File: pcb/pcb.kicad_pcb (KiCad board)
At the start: 2 copper layers, 100 x 115 mm, 27 parts, among them J1 Screw_Terminal_01x02, J2 Screw_Terminal_01x04, J3 Screw_Terminal_01x04, J5 Screw_Terminal_01x06, J6 Screw_Terminal_01x04, Q1 2N7000, Q2 2N7000, Q3 2N7000

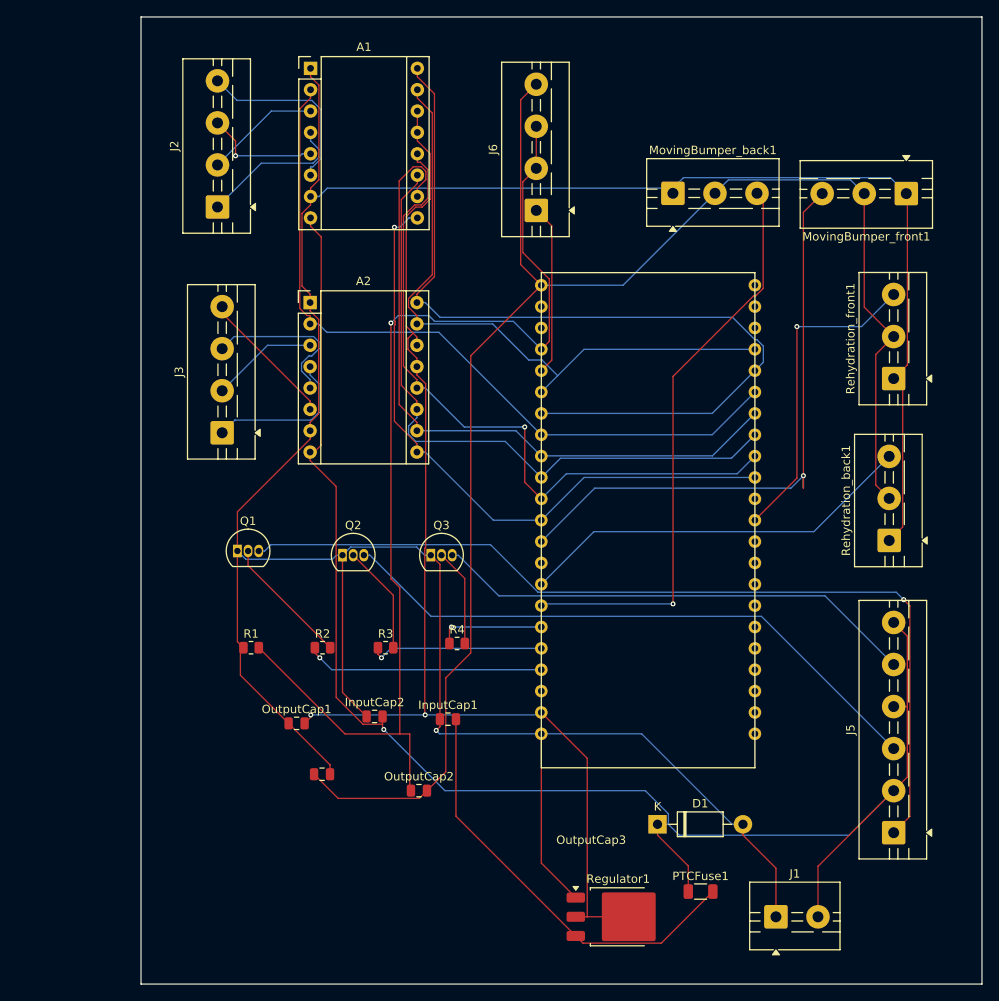
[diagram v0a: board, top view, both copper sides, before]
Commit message: finished layout
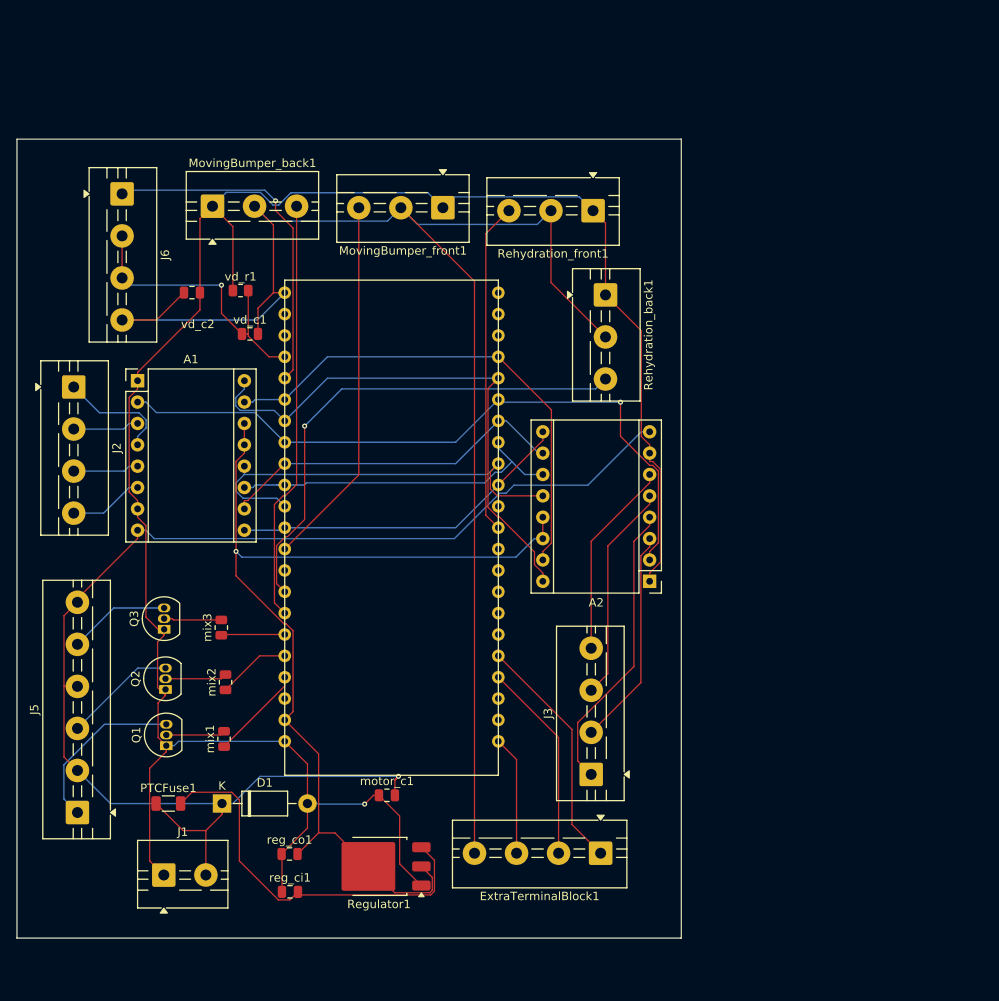
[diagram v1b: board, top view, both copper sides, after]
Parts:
- added ExtraTerminalBlock1: Screw_Terminal_01x04, TerminalBlock:TerminalBlock_MaiXu_MX126-5.0-04P_1x04_P5.00mm, F.Cu at (166.2, 134.4)
- moved J5 97.1 mm to (103.9, 129.6)
- moved J1 73.0 mm to (114.2, 137.0)
- moved PTCFuse1 64.1 mm to (114.8, 128.5)
- moved J3 59.8 mm to (165.0, 125.1)
- moved vd_c2 59.3 mm to (117.6, 67.8)
- moved vd_c1 57.9 mm to (124.5, 72.7)
- moved MovingBumper_front1 55.1 mm to (147.4, 57.7)
- moved MovingBumper_back1 54.8 mm to (120.0, 57.5)
- moved A2 52.2 mm to (172.0, 102.1), turned to 180 degrees
- moved D1 51.8 mm to (121.1, 128.5)
- moved J6 49.3 mm to (109.2, 56.0), turned to -90 degrees
- moved Rehydration_back1 44.6 mm to (166.7, 68.0), turned to -90 degrees
- moved vd_r1 42.5 mm to (123.3, 67.5)
- moved A1 42.5 mm to (111.1, 78.3)
- moved Rehydration_front1 40.9 mm to (165.2, 58.0), turned to 180 degrees
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- renumbered R2 to mix1, R3 to mix2, R4 to mix3, InputCap2 to motor_c1, InputCap1 to reg_ci1, OutputCap1 to reg_co1, OutputCap2 to vd_c1, OutputCap3 to vd_c2, R1 to vd_r1
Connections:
- ESP32-S3 pad 40: unconnected-(ESP32-S3-21-Pad40) -> Net-(ESP32-S3-21)
- ESP32-S3 pad 41: unconnected-(ESP32-S3-20-Pad41) -> Net-(ESP32-S3-20)
- ESP32-S3 pad 44: unconnected-(ESP32-S3-GND-Pad44) -> Net-(ExtraTerminalBlock1-Pin_3)
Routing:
- net Net-(D1-A): track 352.5 -> 254.5 mm
- net /VD_o: track 127.1 -> 35.5 mm
- net Net-(J5-Pin_1): track 108.5 -> 20.5 mm, vias 1 -> 0
- net Net-(J5-Pin_3): track 72.5 -> 13.4 mm
- net Net-(J5-Pin_5): track 57.9 -> 12.1 mm
- net /M0: track 81.6 -> 42.0 mm
- net /DIR: track 103.7 -> 65.0 mm
- net /M1: track 78.2 -> 41.3 mm
- net /EN: track 76.8 -> 40.9 mm, vias 1 -> 0
- net /M2: track 82.5 -> 50.7 mm, vias 1 -> 0
- net /B_F: track 74.8 -> 44.2 mm, vias 1 -> 0
- net Net-(ESP32-S3-21): track 0.00 -> 28.5 mm
- net Net-(A1-VMOT): track 189.6 -> 163.6 mm
- net Net-(ESP32-S3-20): track 0.00 -> 23.9 mm
- net /5V: track 138.9 -> 117.9 mm, vias 2 -> 1
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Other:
- board size 100 x 115 mm -> 79 x 95 mm
